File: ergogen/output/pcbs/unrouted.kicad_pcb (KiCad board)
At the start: 2 copper layers, 220.4 x 89.6 mm, 63 parts

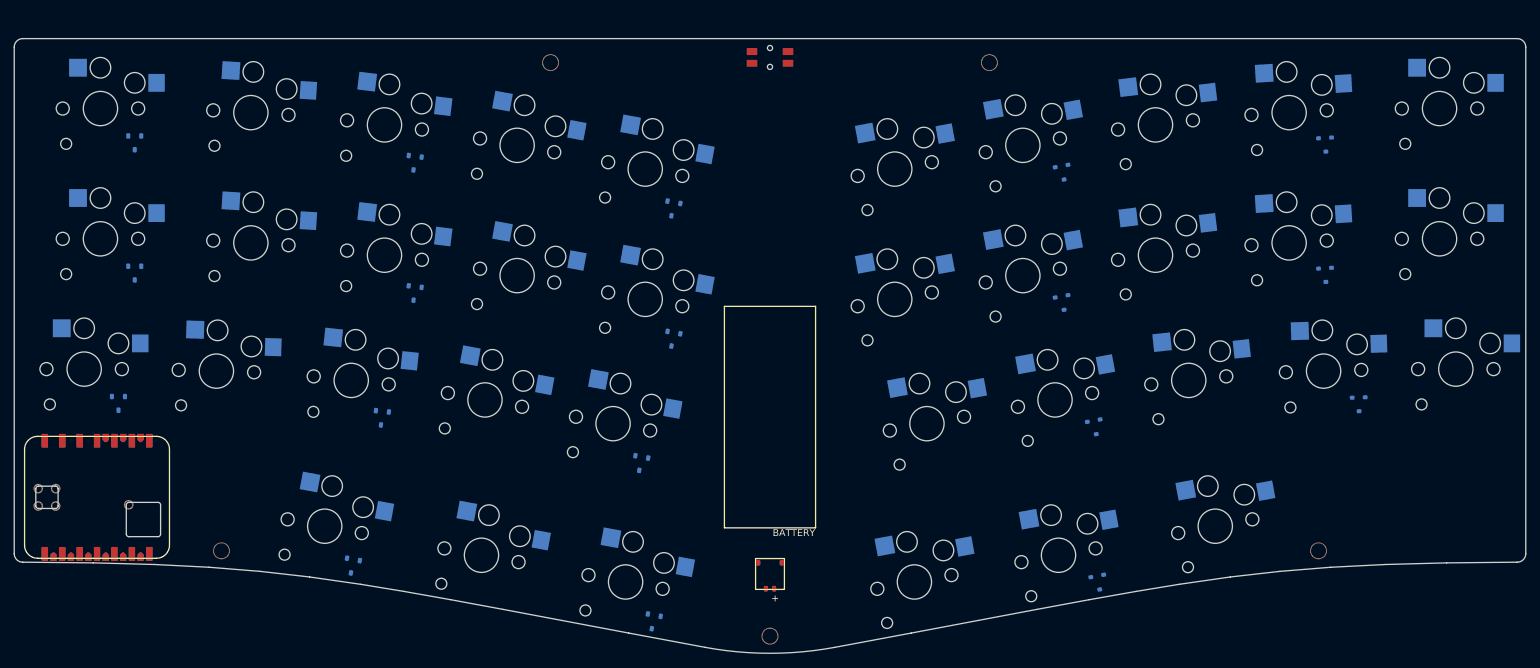
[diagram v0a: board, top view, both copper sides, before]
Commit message: release
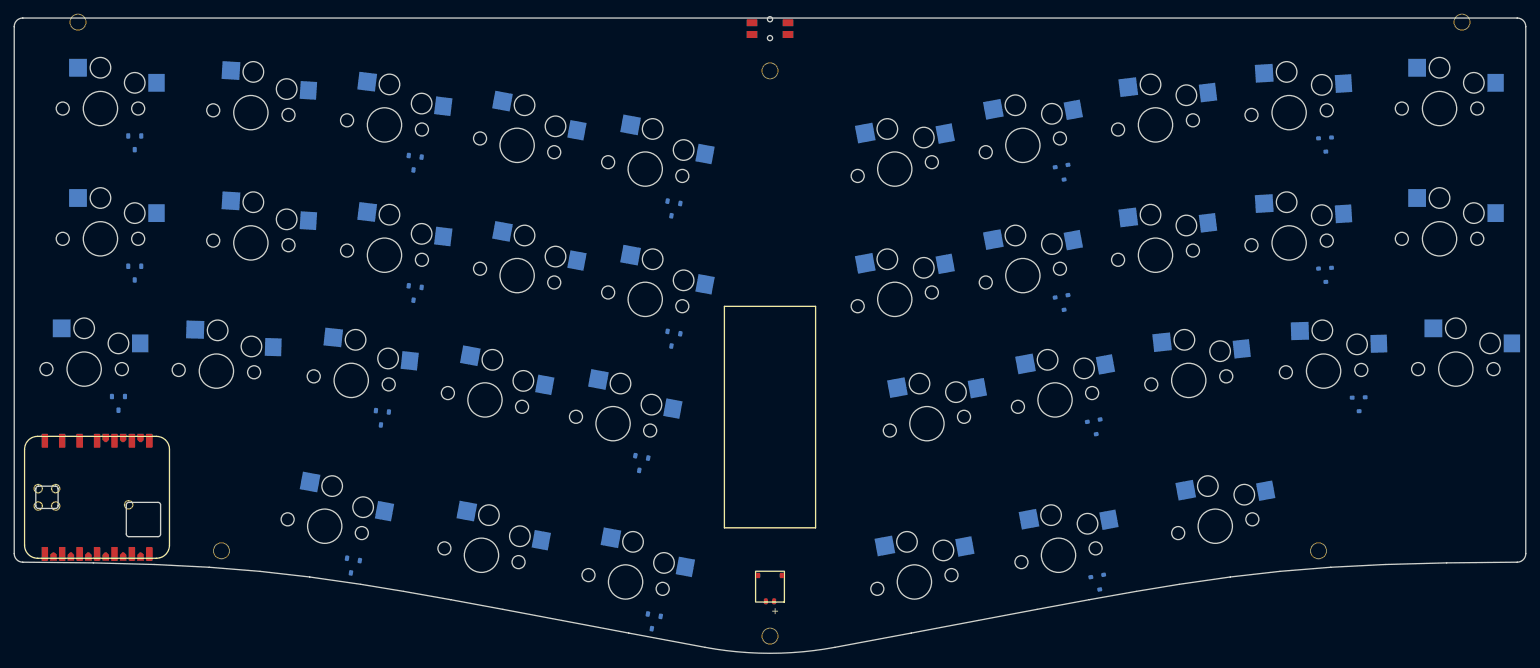
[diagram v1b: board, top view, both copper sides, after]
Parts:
- added H6: , mounting_hole, F.Cu at (177.6, 64.5)
- moved H3 196.7 mm to (198.6, -12.6)
- moved H4 81.0 mm to (17.6, 64.5)
- moved H5 81.0 mm to (97.6, 76.9)
- moved H1 69.2 mm to (-3.28, -12.6)
- moved H2 32.0 mm to (97.6, -5.50)
- moved XX1 4.20 mm to (97.6, -11.7)
- moved XX2 1.85 mm to (97.6, 70.0)
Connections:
- MCU1 pad 3: P0.28 -> C8
- MCU1 pad 4: P0.29 -> C9
- MCU1 pad 5: P0.04 -> C10
- MCU1 pad 6: C8 -> P0.05
- MCU1 pad 7: C10 -> P1.11
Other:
- board size 220.4 x 89.6 mm -> 220.4 x 92.6 mm
- net class Default added: clearance 0.2, trace_width 0.25, via_dia 0.8, via_drill 0.4
- board text removed: "BATTERY"
